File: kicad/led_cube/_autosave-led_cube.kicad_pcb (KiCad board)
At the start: 2 copper layers, 190.5 x 190.5 mm, 76 parts, among them U1 led_cube

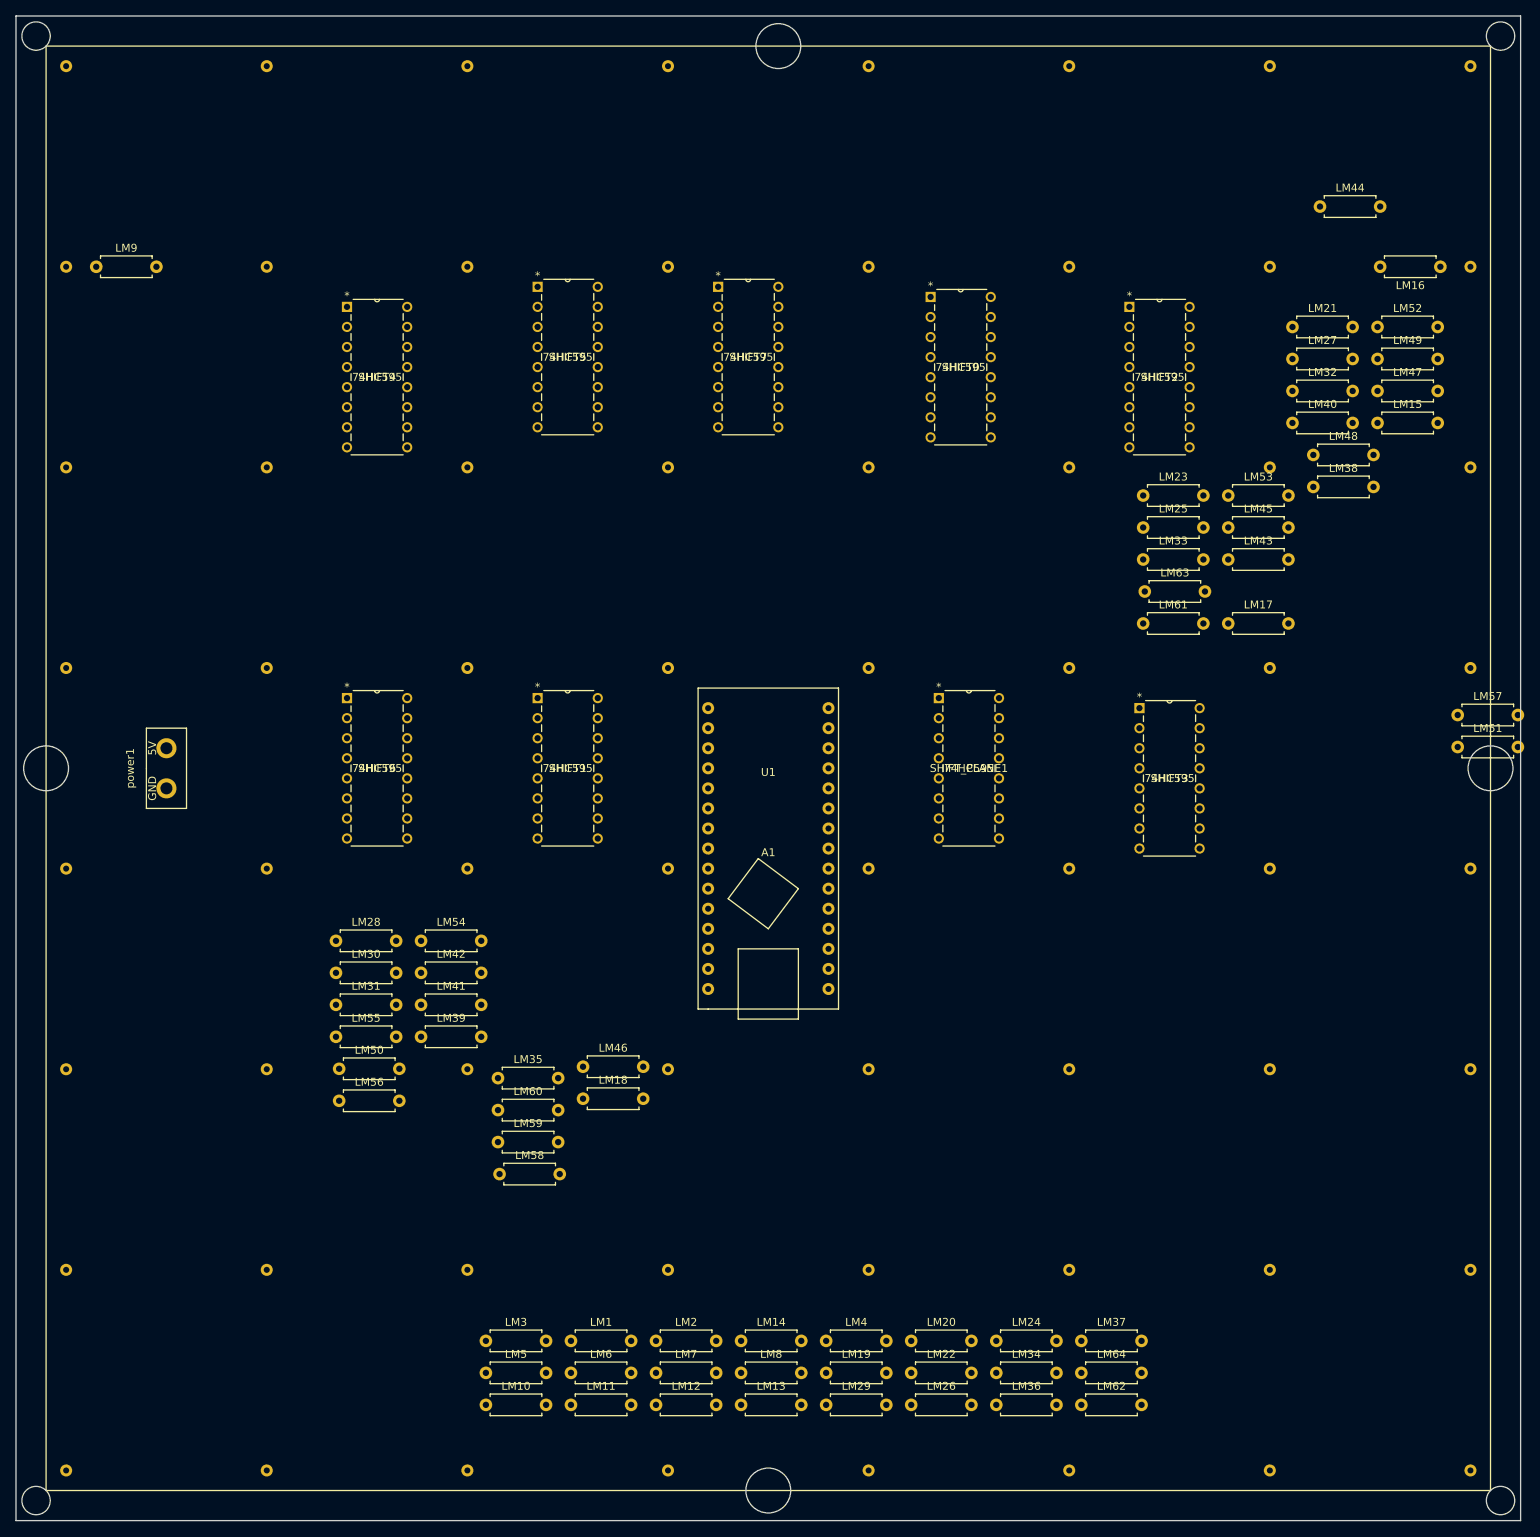
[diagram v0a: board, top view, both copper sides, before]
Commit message: Added lots of stuff
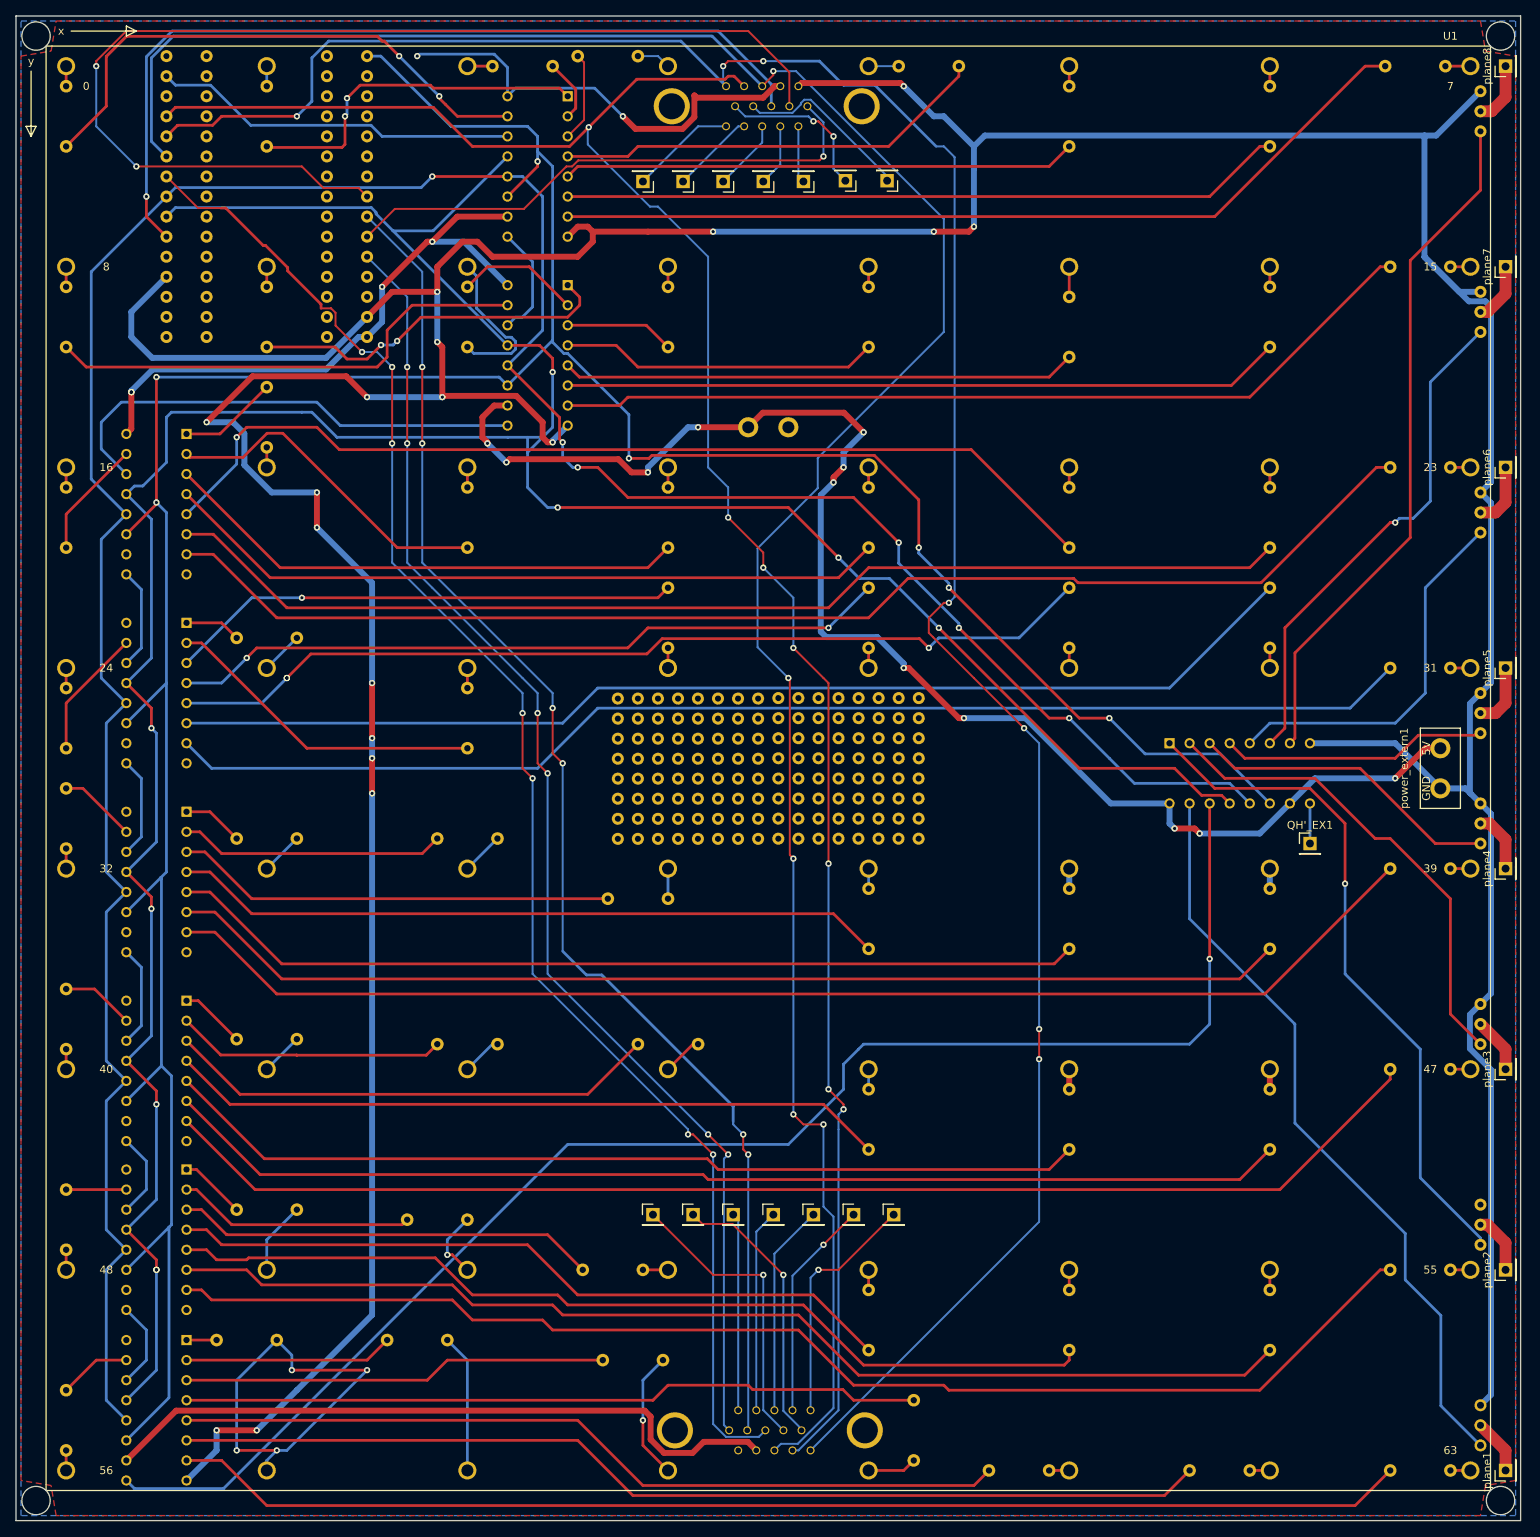
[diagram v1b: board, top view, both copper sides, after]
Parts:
- removed LM1, LM10, LM11, LM12, LM13, LM14, LM15, LM16, LM17, LM18, LM19, LM2, LM20, LM21, LM22, LM23, LM24, LM25, LM26, LM27, LM28, LM29, LM3, LM30, LM31, LM32, LM34, LM35, LM36, LM37, LM38, LM39, LM4, LM40, LM41, LM42, LM43, LM44, LM45, LM46, LM47, LM48, LM49, LM5, LM50, LM51, LM52, LM53, LM54, LM55, LM56, LM57, LM58, LM59, LM6, LM60, LM61, LM62, LM63, LM64, LM7, LM8, LM9: LM, Resistor_THT:R_Axial_DIN0207_L6.3mm_D2.5mm_P7.62mm_Horizontal
- added A2: actual_arduino, footprints:nano, B.Cu at (86.4, 34.3)
- added C1EX1: EX, Connector_PinHeader_2.54mm:PinHeader_1x01_P2.54mm_Vertical, F.Cu at (135.3, 163.2)
- added C1EX2: EX, Connector_PinHeader_2.54mm:PinHeader_1x01_P2.54mm_Vertical, F.Cu at (140.3, 163.2)
- added C1EX3: EX, Connector_PinHeader_2.54mm:PinHeader_1x01_P2.54mm_Vertical, F.Cu at (145.4, 163.2)
- added C1EX4: EX, Connector_PinHeader_2.54mm:PinHeader_1x01_P2.54mm_Vertical, F.Cu at (150.5, 163.2)
- added C1EX5: EX, Connector_PinHeader_2.54mm:PinHeader_1x01_P2.54mm_Vertical, F.Cu at (155.6, 163.2)
- added C1EX6: EX, Connector_PinHeader_2.54mm:PinHeader_1x01_P2.54mm_Vertical, F.Cu at (160.7, 163.2)
- added C1EX7: EX, Connector_PinHeader_2.54mm:PinHeader_1x01_P2.54mm_Vertical, F.Cu at (165.7, 163.2)
- added C2EX1: EX, Connector_PinHeader_2.54mm:PinHeader_1x01_P2.54mm_Vertical, F.Cu at (164.9, 32.3)
- added C2EX2: EX, Connector_PinHeader_2.54mm:PinHeader_1x01_P2.54mm_Vertical, F.Cu at (159.6, 32.3)
- added C2EX3: EX, Connector_PinHeader_2.54mm:PinHeader_1x01_P2.54mm_Vertical, F.Cu at (154.3, 32.4)
- added C2EX4: EX, Connector_PinHeader_2.54mm:PinHeader_1x01_P2.54mm_Vertical, F.Cu at (149.2, 32.4)
- added C2EX5: EX, Connector_PinHeader_2.54mm:PinHeader_1x01_P2.54mm_Vertical, F.Cu at (144.1, 32.4)
- added C2EX6: EX, Connector_PinHeader_2.54mm:PinHeader_1x01_P2.54mm_Vertical, F.Cu at (139.1, 32.4)
- added C2EX7: EX, Connector_PinHeader_2.54mm:PinHeader_1x01_P2.54mm_Vertical, F.Cu at (134.0, 32.4)
- added Controller1: controller, house_cube:15pin_controller, B.Cu at (146.1, 193.0)
- added Controller2: controller, house_cube:15pin_controller, B.Cu at (153.7, 20.3)
- added QH'_EX1: , Connector_PinHeader_2.54mm:PinHeader_1x01_P2.54mm_Vertical, F.Cu at (218.4, 116.2)
- added R1: , Resistor_THT:R_Axial_DIN0207_L6.3mm_D2.5mm_P7.62mm_Horizontal, B.Cu at (86.4, 20.3)
- added R10: , Resistor_THT:R_Axial_DIN0207_L6.3mm_D2.5mm_P7.62mm_Horizontal, B.Cu at (111.8, 53.3)
- added R11: , Resistor_THT:R_Axial_DIN0207_L6.3mm_D2.5mm_P7.62mm_Horizontal, B.Cu at (137.2, 45.7)
- added R12: , Resistor_THT:R_Axial_DIN0207_L6.3mm_D2.5mm_P7.62mm_Horizontal, B.Cu at (162.6, 45.7)
- added R13: , Resistor_THT:R_Axial_DIN0207_L6.3mm_D2.5mm_P7.62mm_Horizontal, B.Cu at (188.0, 47.0)
- added R14: , Resistor_THT:R_Axial_DIN0207_L6.3mm_D2.5mm_P7.62mm_Horizontal, B.Cu at (213.4, 45.7)
- added R15: , Resistor_THT:R_Axial_DIN0207_L6.3mm_D2.5mm_P7.62mm_Horizontal, B.Cu at (236.2, 43.2)
- added R16: , Resistor_THT:R_Axial_DIN0207_L6.3mm_D2.5mm_P7.62mm_Horizontal, B.Cu at (61.0, 71.1)
- added R17: , Resistor_THT:R_Axial_DIN0207_L6.3mm_D2.5mm_P7.62mm_Horizontal, B.Cu at (86.4, 66.0)
- added R18: , Resistor_THT:R_Axial_DIN0207_L6.3mm_D2.5mm_P7.62mm_Horizontal, B.Cu at (111.8, 71.1)
- added R19: , Resistor_THT:R_Axial_DIN0207_L6.3mm_D2.5mm_P7.62mm_Horizontal, B.Cu at (137.2, 71.1)
- added R2: , Resistor_THT:R_Axial_DIN0207_L6.3mm_D2.5mm_P7.62mm_Horizontal, B.Cu at (114.9, 17.8)
- added R20: , Resistor_THT:R_Axial_DIN0207_L6.3mm_D2.5mm_P7.62mm_Horizontal, B.Cu at (162.6, 71.1)
- added R21: , Resistor_THT:R_Axial_DIN0207_L6.3mm_D2.5mm_P7.62mm_Horizontal, B.Cu at (188.0, 71.1)
- added R22: , Resistor_THT:R_Axial_DIN0207_L6.3mm_D2.5mm_P7.62mm_Horizontal, B.Cu at (213.4, 71.1)
- added R23: , Resistor_THT:R_Axial_DIN0207_L6.3mm_D2.5mm_P7.62mm_Horizontal, B.Cu at (236.2, 68.6)
- added R24: , Resistor_THT:R_Axial_DIN0207_L6.3mm_D2.5mm_P7.62mm_Horizontal, B.Cu at (61.0, 96.5)
- added R25: , Resistor_THT:R_Axial_DIN0207_L6.3mm_D2.5mm_P7.62mm_Horizontal, B.Cu at (90.2, 90.2)
- added R26: , Resistor_THT:R_Axial_DIN0207_L6.3mm_D2.5mm_P7.62mm_Horizontal, B.Cu at (111.8, 96.5)
- added R27: , Resistor_THT:R_Axial_DIN0207_L6.3mm_D2.5mm_P7.62mm_Horizontal, B.Cu at (137.2, 91.4)
- added R28: , Resistor_THT:R_Axial_DIN0207_L6.3mm_D2.5mm_P7.62mm_Horizontal, B.Cu at (162.6, 91.4)
- added R29: , Resistor_THT:R_Axial_DIN0207_L6.3mm_D2.5mm_P7.62mm_Horizontal, B.Cu at (188.0, 91.4)
- added R3: , Resistor_THT:R_Axial_DIN0207_L6.3mm_D2.5mm_P7.62mm_Horizontal, B.Cu at (133.3, 16.5)
- added R30: , Resistor_THT:R_Axial_DIN0207_L6.3mm_D2.5mm_P7.62mm_Horizontal, B.Cu at (213.4, 91.4)
- added R31: , Resistor_THT:R_Axial_DIN0207_L6.3mm_D2.5mm_P7.62mm_Horizontal, B.Cu at (236.2, 94.0)
- added R32: , Resistor_THT:R_Axial_DIN0207_L6.3mm_D2.5mm_P7.62mm_Horizontal, B.Cu at (61.0, 116.8)
- added R33: , Resistor_THT:R_Axial_DIN0207_L6.3mm_D2.5mm_P7.62mm_Horizontal, B.Cu at (90.2, 115.6)
- added R34: , Resistor_THT:R_Axial_DIN0207_L6.3mm_D2.5mm_P7.62mm_Horizontal, B.Cu at (115.6, 115.6)
- added R35: , Resistor_THT:R_Axial_DIN0207_L6.3mm_D2.5mm_P7.62mm_Horizontal, B.Cu at (137.2, 123.2)
- added R36: , Resistor_THT:R_Axial_DIN0207_L6.3mm_D2.5mm_P7.62mm_Horizontal, B.Cu at (162.6, 121.9)
- added R37: , Resistor_THT:R_Axial_DIN0207_L6.3mm_D2.5mm_P7.62mm_Horizontal, B.Cu at (188.0, 121.9)
- added R38: , Resistor_THT:R_Axial_DIN0207_L6.3mm_D2.5mm_P7.62mm_Horizontal, B.Cu at (213.4, 121.9)
- added R39: , Resistor_THT:R_Axial_DIN0207_L6.3mm_D2.5mm_P7.62mm_Horizontal, B.Cu at (236.2, 119.4)
- added R4: , Resistor_THT:R_Axial_DIN0207_L6.3mm_D2.5mm_P7.62mm_Horizontal, B.Cu at (166.4, 17.8)
- added R40: , Resistor_THT:R_Axial_DIN0207_L6.3mm_D2.5mm_P7.62mm_Horizontal, B.Cu at (61.0, 142.2)
- added R41: , Resistor_THT:R_Axial_DIN0207_L6.3mm_D2.5mm_P7.62mm_Horizontal, B.Cu at (90.2, 141.0)
- added R42: , Resistor_THT:R_Axial_DIN0207_L6.3mm_D2.5mm_P7.62mm_Horizontal, B.Cu at (115.6, 141.6)
- added R43: , Resistor_THT:R_Axial_DIN0207_L6.3mm_D2.5mm_P7.62mm_Horizontal, B.Cu at (141.0, 141.6)
- added R44: , Resistor_THT:R_Axial_DIN0207_L6.3mm_D2.5mm_P7.62mm_Horizontal, B.Cu at (162.6, 147.3)
- added R45: , Resistor_THT:R_Axial_DIN0207_L6.3mm_D2.5mm_P7.62mm_Horizontal, B.Cu at (188.0, 147.3)
- added R46: , Resistor_THT:R_Axial_DIN0207_L6.3mm_D2.5mm_P7.62mm_Horizontal, B.Cu at (213.4, 147.3)
- added R47: , Resistor_THT:R_Axial_DIN0207_L6.3mm_D2.5mm_P7.62mm_Horizontal, B.Cu at (236.2, 144.8)
- added R48: , Resistor_THT:R_Axial_DIN0207_L6.3mm_D2.5mm_P7.62mm_Horizontal, B.Cu at (61.0, 167.6)
- added R49: , Resistor_THT:R_Axial_DIN0207_L6.3mm_D2.5mm_P7.62mm_Horizontal, B.Cu at (90.2, 162.6)
- added R5: , Resistor_THT:R_Axial_DIN0207_L6.3mm_D2.5mm_P7.62mm_Horizontal, B.Cu at (188.0, 20.3)
- added R50: , Resistor_THT:R_Axial_DIN0207_L6.3mm_D2.5mm_P7.62mm_Horizontal, B.Cu at (111.8, 163.8)
- added R51: , Resistor_THT:R_Axial_DIN0207_L6.3mm_D2.5mm_P7.62mm_Horizontal, B.Cu at (134.0, 170.2)
- added R52: , Resistor_THT:R_Axial_DIN0207_L6.3mm_D2.5mm_P7.62mm_Horizontal, B.Cu at (162.6, 172.7)
- added R53: , Resistor_THT:R_Axial_DIN0207_L6.3mm_D2.5mm_P7.62mm_Horizontal, B.Cu at (188.0, 172.7)
- added R54: , Resistor_THT:R_Axial_DIN0207_L6.3mm_D2.5mm_P7.62mm_Horizontal, B.Cu at (213.4, 172.7)
- added R55: , Resistor_THT:R_Axial_DIN0207_L6.3mm_D2.5mm_P7.62mm_Horizontal, B.Cu at (236.2, 170.2)
- added R56: , Resistor_THT:R_Axial_DIN0207_L6.3mm_D2.5mm_P7.62mm_Horizontal, B.Cu at (61.0, 193.0)
- added R57: , Resistor_THT:R_Axial_DIN0207_L6.3mm_D2.5mm_P7.62mm_Horizontal, B.Cu at (87.6, 179.1)
- added R58: , Resistor_THT:R_Axial_DIN0207_L6.3mm_D2.5mm_P7.62mm_Horizontal, B.Cu at (109.2, 179.1)
- added R59: , Resistor_THT:R_Axial_DIN0207_L6.3mm_D2.5mm_P7.62mm_Horizontal, B.Cu at (136.5, 181.6)
- added R6: , Resistor_THT:R_Axial_DIN0207_L6.3mm_D2.5mm_P7.62mm_Horizontal, B.Cu at (213.4, 20.3)
- added R60: , Resistor_THT:R_Axial_DIN0207_L6.3mm_D2.5mm_P7.62mm_Horizontal, B.Cu at (168.3, 194.3)
- added R61: , Resistor_THT:R_Axial_DIN0207_L6.3mm_D2.5mm_P7.62mm_Horizontal, B.Cu at (185.4, 195.6)
- added R62: , Resistor_THT:R_Axial_DIN0207_L6.3mm_D2.5mm_P7.62mm_Horizontal, B.Cu at (210.8, 195.6)
- added R63: , Resistor_THT:R_Axial_DIN0207_L6.3mm_D2.5mm_P7.62mm_Horizontal, B.Cu at (236.2, 195.6)
- added R7: , Resistor_THT:R_Axial_DIN0207_L6.3mm_D2.5mm_P7.62mm_Horizontal, B.Cu at (235.6, 17.8)
- added R8: , Resistor_THT:R_Axial_DIN0207_L6.3mm_D2.5mm_P7.62mm_Horizontal, B.Cu at (61.0, 45.7)
- added R9: , Resistor_THT:R_Axial_DIN0207_L6.3mm_D2.5mm_P7.62mm_Horizontal, B.Cu at (86.4, 45.7)
- added _1: _, house_cube:proto, F.Cu at (151.1, 105.4)
- added _2: _, house_cube:proto, F.Cu at (161.3, 105.4)
- added _3: _, house_cube:proto, F.Cu at (151.1, 115.6)
- added _4: _, house_cube:proto, F.Cu at (161.3, 115.6)
- added _5: _, house_cube:proto, F.Cu at (130.8, 115.6)
- added _6: _, house_cube:proto, F.Cu at (140.9, 115.6)
- added _7: _, house_cube:proto, F.Cu at (130.8, 105.5)
- added _8: _, house_cube:proto, F.Cu at (140.9, 105.5)
- added fet1: gen_mosfet, house_cube:gen_fet, B.Cu at (240.0, 189.9)
- added fet2: gen_mosfet, house_cube:gen_fet, B.Cu at (240.0, 164.5)
- added fet3: gen_mosfet, house_cube:gen_fet, B.Cu at (240.0, 139.1)
- added fet4: gen_mosfet, house_cube:gen_fet, B.Cu at (240.0, 113.7)
- added fet5: gen_mosfet, house_cube:gen_fet, B.Cu at (240.0, 99.7)
- added fet6: gen_mosfet, house_cube:gen_fet, B.Cu at (240.0, 74.3)
- added fet7: gen_mosfet, house_cube:gen_fet, B.Cu at (240.0, 48.9)
- added fet8: gen_mosfet, house_cube:gen_fet, B.Cu at (240.0, 23.5)
- added plane1: , Connector_PinHeader_2.54mm:PinHeader_1x01_P2.54mm_Vertical, F.Cu at (243.2, 195.6)
- added plane2: , Connector_PinHeader_2.54mm:PinHeader_1x01_P2.54mm_Vertical, F.Cu at (243.2, 170.2)
- added plane3: , Connector_PinHeader_2.54mm:PinHeader_1x01_P2.54mm_Vertical, F.Cu at (243.2, 144.8)
- added plane4: , Connector_PinHeader_2.54mm:PinHeader_1x01_P2.54mm_Vertical, F.Cu at (243.2, 119.4)
- added plane5: , Connector_PinHeader_2.54mm:PinHeader_1x01_P2.54mm_Vertical, F.Cu at (243.2, 94.0)
- added plane6: , Connector_PinHeader_2.54mm:PinHeader_1x01_P2.54mm_Vertical, F.Cu at (243.2, 68.6)
- added plane7: , Connector_PinHeader_2.54mm:PinHeader_1x01_P2.54mm_Vertical, F.Cu at (243.2, 43.2)
- added plane8: , Connector_PinHeader_2.54mm:PinHeader_1x01_P2.54mm_Vertical, F.Cu at (243.2, 17.8)
- added power_extern1: power, footprints:power, F.Cu at (234.9, 106.7)
- A1: value Arduino_Nano_v3.x -> arduino_buffer; footprint footprints:nano -> house_cube:nano_buffer; moved to B.Cu
- R0: renamed from LM33; value LM -> (none); moved to B.Cu
- SHIFT0, SHIFT1, SHIFT2, SHIFT3, SHIFT4, SHIFT5, SHIFT6, SHIFT7, SHIFT_PLANE1, power1: moved to B.Cu
- moved SHIFT7 156.8 mm to (68.6, 196.8), turned to 180 degrees
- moved R0 149.0 mm to (61.0, 20.3), turned to 270 degrees
- moved SHIFT3 136.3 mm to (68.6, 106.0), turned to 180 degrees
- moved SHIFT2 135.6 mm to (68.6, 82.1), turned to 180 degrees
- moved SHIFT5 108.3 mm to (68.6, 153.9), turned to 180 degrees
- moved A1 104.1 mm to (86.4, 34.3)
- moved power1 87.6 mm to (149.9, 63.5), turned to 180 degrees
- moved SHIFT4 73.1 mm to (68.6, 130.0), turned to 180 degrees
- moved SHIFT6 69.5 mm to (68.6, 175.3), turned to 180 degrees
- moved SHIFT0 66.3 mm to (116.8, 39.4), turned to 180 degrees
- moved SHIFT1 53.5 mm to (116.8, 63.3), turned to 180 degrees
- moved SHIFT_PLANE1 39.6 mm to (218.4, 111.1), turned to 270 degrees
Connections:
- A1 pad 1: Net-(A1-Pad1) -> (no net)
- A1 pad 10: Net-(A1-Pad10) -> BUTTON_CLOCK
- A1 pad 11: Net-(A1-Pad11) -> BUTTON_LATCH
- A1 pad 12: Net-(A1-Pad12) -> BUTTON_DATA
- A1 pad 13: Net-(A1-Pad13) -> (no net)
- A1 pad 14: Net-(A1-Pad14) -> data
- A1 pad 15: Net-(A1-Pad15) -> (no net)
- A1 pad 16: Net-(A1-Pad16) -> srclk
- A1 pad 17: Net-(A1-Pad17) -> (no net)
- A1 pad 18: Net-(A1-Pad18) -> (no net)
- A1 pad 19: Net-(A1-Pad19) -> (no net)
- A1 pad 2: Net-(A1-Pad2) -> (no net)
- A1 pad 20: Net-(A1-Pad20) -> (no net)
- A1 pad 21: Net-(A1-Pad21) -> (no net)
- A1 pad 22: Net-(A1-Pad22) -> (no net)
- A1 pad 23: Net-(A1-Pad23) -> JOY_V2
- A1 pad 24: Net-(A1-Pad24) -> JOY_V1
- A1 pad 25: Net-(A1-Pad25) -> JOY_H2
- A1 pad 26: Net-(A1-Pad26) -> JOY_H1
- A1 pad 27: Net-(A1-Pad27) -> (no net)
- A1 pad 28: Net-(A1-Pad28) -> (no net)
- A1 pad 29: Net-(A1-Pad29) -> GND
- A1 pad 3: Net-(A1-Pad3) -> (no net)
- A1 pad 30: Net-(A1-Pad30) -> +5V
- A1 pad 4: Net-(A1-Pad4) -> GND
- A1 pad 5: Net-(A1-Pad5) -> (no net)
- A1 pad 6: Net-(A1-Pad6) -> BUTTON_WATCH2
- A1 pad 7: srclk -> output_enable
- A1 pad 9: d6 -> BUTTON_WATCH1
- R0 pad 1: led43 -> Net-(R0-Pad1)
- R0 pad 2: Net-(LM33-Pad2) -> led0
- SHIFT0 pad 13: GND -> output_enable
- SHIFT0 pad 14: d6 -> data
- SHIFT1 pad 13: GND -> output_enable
- SHIFT2 pad 13: GND -> output_enable
- SHIFT3 pad 13: GND -> output_enable
- SHIFT4 pad 13: GND -> output_enable
- SHIFT5 pad 13: GND -> output_enable
- SHIFT6 pad 13: GND -> output_enable
- SHIFT7 pad 13: GND -> output_enable
- SHIFT_PLANE1 pad 1: plane1 -> pg1
- SHIFT_PLANE1 pad 13: GND -> output_enable
- SHIFT_PLANE1 pad 14: Net-(SHIFT_PLANE1-Pad14) -> Net-(SHIFT7-Pad9)
- SHIFT_PLANE1 pad 15: plane0 -> pg0
- SHIFT_PLANE1 pad 2: plane2 -> pg2
- SHIFT_PLANE1 pad 3: plane3 -> pg3
- SHIFT_PLANE1 pad 4: plane4 -> pg4
- SHIFT_PLANE1 pad 5: plane5 -> pg5
- SHIFT_PLANE1 pad 6: plane6 -> pg6
- SHIFT_PLANE1 pad 7: plane7 -> pg7
- SHIFT_PLANE1 pad 9: Net-(SHIFT7-Pad9) -> Net-(QH'_EX1-Pad1)
- U1 pad 0: Net-(LM1-Pad1) -> Net-(R0-Pad1)
- U1 pad 63: Net-(LM33-Pad2) -> Net-(R63-Pad1)
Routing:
- net GND: track 0.00 -> 666.7 mm, vias 0 -> 18
- net srclk: track 0.00 -> 407.0 mm, vias 0 -> 7
- net +5V: track 0.00 -> 405.4 mm, vias 0 -> 18
- net output_enable: track 0.00 -> 391.9 mm, vias 0 -> 9
- net rclk: track 0.00 -> 366.3 mm, vias 0 -> 6
- net BUTTON_LATCH: track 0.00 -> 302.0 mm, vias 0 -> 7
- net BUTTON_CLOCK: track 0.00 -> 301.7 mm, vias 0 -> 5
- net BUTTON_DATA: track 0.00 -> 264.8 mm, vias 0 -> 7
- net BUTTON_WATCH1: track 0.00 -> 198.7 mm, vias 0 -> 7
- net Net-(SHIFT7-Pad9): track 0.00 -> 191.7 mm, vias 0 -> 1
- net JOY_V1: track 0.00 -> 174.9 mm, vias 0 -> 6
- net JOY_H1: track 0.00 -> 168.0 mm, vias 0 -> 6
- net led23: track 0.00 -> 164.1 mm
- net led55: track 0.00 -> 164.0 mm
- net led47: track 0.00 -> 163.1 mm
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- added copper zone on F.Cu, net +5V
- added copper zone on B.Cu, net GND
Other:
- outline, holes or cut-outs redrawn
- board text added: "Hello person"
- board text added: "x"
- board text added: "y"
